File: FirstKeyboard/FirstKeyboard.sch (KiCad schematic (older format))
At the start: 24 parts, among them J1 USB_B_Mini, SW1 MXSwitch, SW2 MXSwitch, SW3 MXSwitch, SW4 MXSwitch, U1 ATmega32U4-AU, Y1 16MHz

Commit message: Last update of the day
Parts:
- C1, C2, C3, C4, C5, C6, C7, C8: footprint (none) -> Capacitor_SMD:C_0805_2012Metric_Pad1.15x1.40mm_HandSolder
- D1, D2, D3, D4: footprint (none) -> Diode_SMD:D_SOD-123
- J1: footprint (none) -> acheron_Connectors:USB_MiniB_XM7D-0512
- R1, R2, R3, R4: footprint (none) -> Resistor_SMD:R_1206_3216Metric_Pad1.42x1.75mm_HandSolder
- SW1, SW2, SW3, SW4: footprint (none) -> acheron_MX:MX100
- SWP1: footprint (none) -> acheron_Hardware:smdPushBtn
- Y1: footprint (none) -> Crystal:Crystal_SMD_5032-2Pin_5.0x3.2mm_HandSoldering
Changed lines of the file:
@@
 F 0 "SW1" H 7000 3000 50  0000 L CNN
 F 1 "MXSwitch" H 6950 2925 39  0000 L CNN
-F 2 "" H 7075 2925 50  0001 C CNN
+F 2 "acheron_MX:MX100" H 7075 2925 50  0001 C CNN
 F 3 "" H 7075 2925 50  0001 C CNN
 	1    7075 2925
@@
 F 0 "D1" V 7029 2543 50  0000 L CNN
 F 1 "D_Small" V 7120 2543 50  0000 L CNN
-F 2 "" V 7075 2475 50  0001 C CNN
+F 2 "Diode_SMD:D_SOD-123" V 7075 2475 50  0001 C CNN
 F 3 "~" V 7075 2475 50  0001 C CNN
 	1    7075 2475
@@
 F 0 "SW3" H 7925 3000 50  0000 L CNN
 F 1 "MXSwitch" H 7875 2925 39  0000 L CNN
-F 2 "" H 8000 2925 50  0001 C CNN
+F 2 "acheron_MX:MX100" H 8000 2925 50  0001 C CNN
 F 3 "" H 8000 2925 50  0001 C CNN
 	1    8000 2925
@@
 F 0 "D3" V 7954 2543 50  0000 L CNN
 F 1 "D_Small" V 8045 2543 50  0000 L CNN
-F 2 "" V 8000 2475 50  0001 C CNN
+F 2 "Diode_SMD:D_SOD-123" V 8000 2475 50  0001 C CNN
 F 3 "~" V 8000 2475 50  0001 C CNN
 	1    8000 2475
@@
 F 0 "SW4" H 7925 4275 50  0000 L CNN
 F 1 "MXSwitch" H 7875 4200 39  0000 L CNN
-F 2 "" H 8000 4200 50  0001 C CNN
+F 2 "acheron_MX:MX100" H 8000 4200 50  0001 C CNN
 F 3 "" H 8000 4200 50  0001 C CNN
 	1    8000 4200
@@
 F 0 "D4" V 7954 3818 50  0000 L CNN
 F 1 "D_Small" V 8045 3818 50  0000 L CNN
-F 2 "" V 8000 3750 50  0001 C CNN
+F 2 "Diode_SMD:D_SOD-123" V 8000 3750 50  0001 C CNN
 F 3 "~" V 8000 3750 50  0001 C CNN
 	1    8000 3750
@@
 F 0 "SW2" H 7000 4275 50  0000 L CNN
 F 1 "MXSwitch" H 6950 4200 39  0000 L CNN
-F 2 "" H 7075 4200 50  0001 C CNN
+F 2 "acheron_MX:MX100" H 7075 4200 50  0001 C CNN
 F 3 "" H 7075 4200 50  0001 C CNN
 	1    7075 4200
@@
 F 0 "D2" V 7029 3818 50  0000 L CNN
 F 1 "D_Small" V 7120 3818 50  0000 L CNN
-F 2 "" V 7075 3750 50  0001 C CNN
+F 2 "Diode_SMD:D_SOD-123" V 7075 3750 50  0001 C CNN
 F 3 "~" V 7075 3750 50  0001 C CNN
 	1    7075 3750
@@
 F 0 "R3" V 2604 5000 50  0000 C CNN
 F 1 "22R" V 2695 5000 50  0000 C CNN
-F 2 "" H 2800 5000 50  0001 C CNN
+F 2 "Resistor_SMD:R_1206_3216Metric_Pad1.42x1.75mm_HandSolder" H 2800 5000 50  0001 C CNN
 F 3 "~" H 2800 5000 50  0001 C CNN
 	1    2800 5000
@@
 F 0 "R2" V 2604 4900 50  0000 C CNN
 F 1 "22R" V 2695 4900 50  0000 C CNN
-F 2 "" H 2800 4900 50  0001 C CNN
+F 2 "Resistor_SMD:R_1206_3216Metric_Pad1.42x1.75mm_HandSolder" H 2800 4900 50  0001 C CNN
 F 3 "~" H 2800 4900 50  0001 C CNN
 	1    2800 4900
@@
 F 0 "J1" H 2150 5375 50  0000 C CNN
 F 1 "USB_B_Mini" H 2150 5275 50  0000 C CNN
-F 2 "" H 2300 4850 50  0001 C CNN
+F 2 "acheron_Connectors:USB_MiniB_XM7D-0512" H 2300 4850 50  0001 C CNN
 F 3 "~" H 2300 4850 50  0001 C CNN
 	1    2150 4900
@@
 F 0 "C5" V 3825 2575 50  0000 C CNN
 F 1 "10uF" V 3725 2575 50  0000 C CNN
-F 2 "" H 3625 2575 50  0001 C CNN
+F 2 "Capacitor_SMD:C_0805_2012Metric_Pad1.15x1.40mm_HandSolder" H 3625 2575 50  0001 C CNN
 F 3 "~" H 3625 2575 50  0001 C CNN
 	1    3625 2575
@@
 F 0 "C6" V 4125 2575 50  0000 C CNN
 F 1 "1uF" V 4025 2575 50  0000 C CNN
-F 2 "" H 3925 2575 50  0001 C CNN
+F 2 "Capacitor_SMD:C_0805_2012Metric_Pad1.15x1.40mm_HandSolder" H 3925 2575 50  0001 C CNN
 F 3 "~" H 3925 2575 50  0001 C CNN
 	1    3925 2575
@@
 F 0 "C7" V 4425 2575 50  0000 C CNN
 F 1 "100n" V 4325 2575 50  0000 C CNN
-F 2 "" H 4225 2575 50  0001 C CNN
+F 2 "Capacitor_SMD:C_0805_2012Metric_Pad1.15x1.40mm_HandSolder" H 4225 2575 50  0001 C CNN
 F 3 "~" H 4225 2575 50  0001 C CNN
 	1    4225 2575
@@
 F 0 "C8" V 4725 2575 50  0000 C CNN
 F 1 "100n" V 4625 2575 50  0000 C CNN
-F 2 "" H 4525 2575 50  0001 C CNN
+F 2 "Capacitor_SMD:C_0805_2012Metric_Pad1.15x1.40mm_HandSolder" H 4525 2575 50  0001 C CNN
 F 3 "~" H 4525 2575 50  0001 C CNN
 	1    4525 2575
@@
 F 0 "R1" H 2716 2854 50  0000 R CNN
 F 1 "10k" H 2716 2945 50  0000 R CNN
-F 2 "" H 2775 2900 50  0001 C CNN
+F 2 "Resistor_SMD:R_1206_3216Metric_Pad1.42x1.75mm_HandSolder" H 2775 2900 50  0001 C CNN
 F 3 "~" H 2775 2900 50  0001 C CNN
 	1    2775 2900
@@
 F 0 "SWP1" H 2700 3550 50  0000 R CNN
 F 1 "SW_Push" H 2725 3450 50  0000 R CNN
-F 2 "" H 2575 3400 50  0001 C CNN
+F 2 "acheron_Hardware:smdPushBtn" H 2575 3400 50  0001 C CNN
 F 3 "~" H 2575 3400 50  0001 C CNN
 	1    2575 3200
@@
 F 0 "C1" H 3025 3100 50  0000 R CNN
 F 1 "100n" H 3075 3300 50  0000 R CNN
-F 2 "" H 3075 3200 50  0001 C CNN
+F 2 "Capacitor_SMD:C_0805_2012Metric_Pad1.15x1.40mm_HandSolder" H 3075 3200 50  0001 C CNN
 F 3 "~" H 3075 3200 50  0001 C CNN
 	1    3075 3200
@@
 F 0 "R4" V 4729 6000 50  0000 C CNN
 F 1 "10k" V 4820 6000 50  0000 C CNN
-F 2 "" H 4925 6000 50  0001 C CNN
+F 2 "Resistor_SMD:R_1206_3216Metric_Pad1.42x1.75mm_HandSolder" H 4925 6000 50  0001 C CNN
 F 3 "~" H 4925 6000 50  0001 C CNN
 	1    4925 6000
@@
 F 0 "C3" V 2896 4300 50  0000 C CNN
 F 1 "22pF" V 2987 4300 50  0000 C CNN
-F 2 "" H 3125 4300 50  0001 C CNN
+F 2 "Capacitor_SMD:C_0805_2012Metric_Pad1.15x1.40mm_HandSolder" H 3125 4300 50  0001 C CNN
 F 3 "~" H 3125 4300 50  0001 C CNN
 	1    3125 4300
@@
 F 0 "C2" V 2975 4250 50  0000 C CNN
 F 1 "22pF" V 2987 4100 50  0000 C CNN
-F 2 "" H 3125 4100 50  0001 C CNN
+F 2 "Capacitor_SMD:C_0805_2012Metric_Pad1.15x1.40mm_HandSolder" H 3125 4100 50  0001 C CNN
 F 3 "~" H 3125 4100 50  0001 C CNN
 	1    3125 4100
@@
 F 0 "Y1" V 3225 4250 50  0000 R CNN
 F 1 "16MHz" V 3125 4300 50  0000 R CNN
-F 2 "" H 3375 4200 50  0001 C CNN
+F 2 "Crystal:Crystal_SMD_5032-2Pin_5.0x3.2mm_HandSoldering" H 3375 4200 50  0001 C CNN
 F 3 "~" H 3375 4200 50  0001 C CNN
 	1    3375 4200
@@
 F 0 "C4" V 3575 5200 50  0000 C CNN
 F 1 "1uF" V 3675 5200 50  0000 C CNN
-F 2 "" H 3425 5200 50  0001 C CNN
+F 2 "Capacitor_SMD:C_0805_2012Metric_Pad1.15x1.40mm_HandSolder" H 3425 5200 50  0001 C CNN
 F 3 "~" H 3425 5200 50  0001 C CNN
 	1    3425 5200

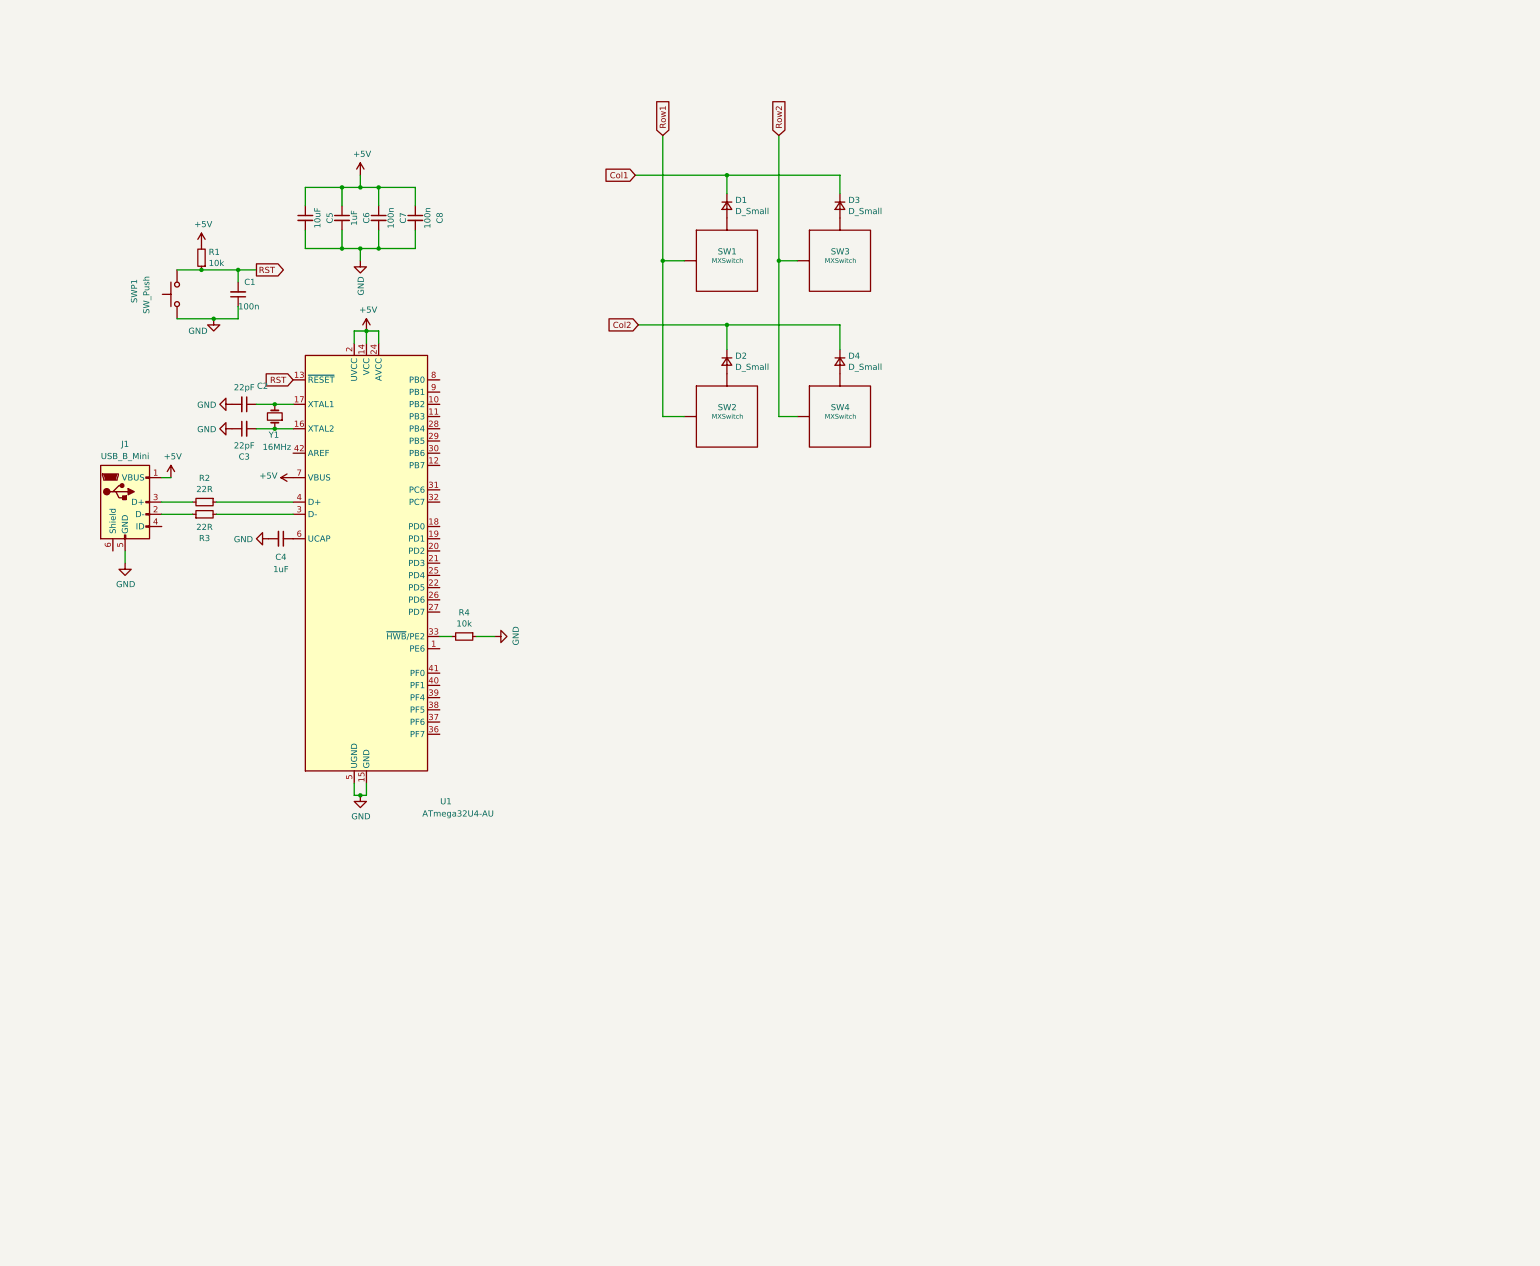
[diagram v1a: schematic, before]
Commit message: Dec10 Update, Starting full board
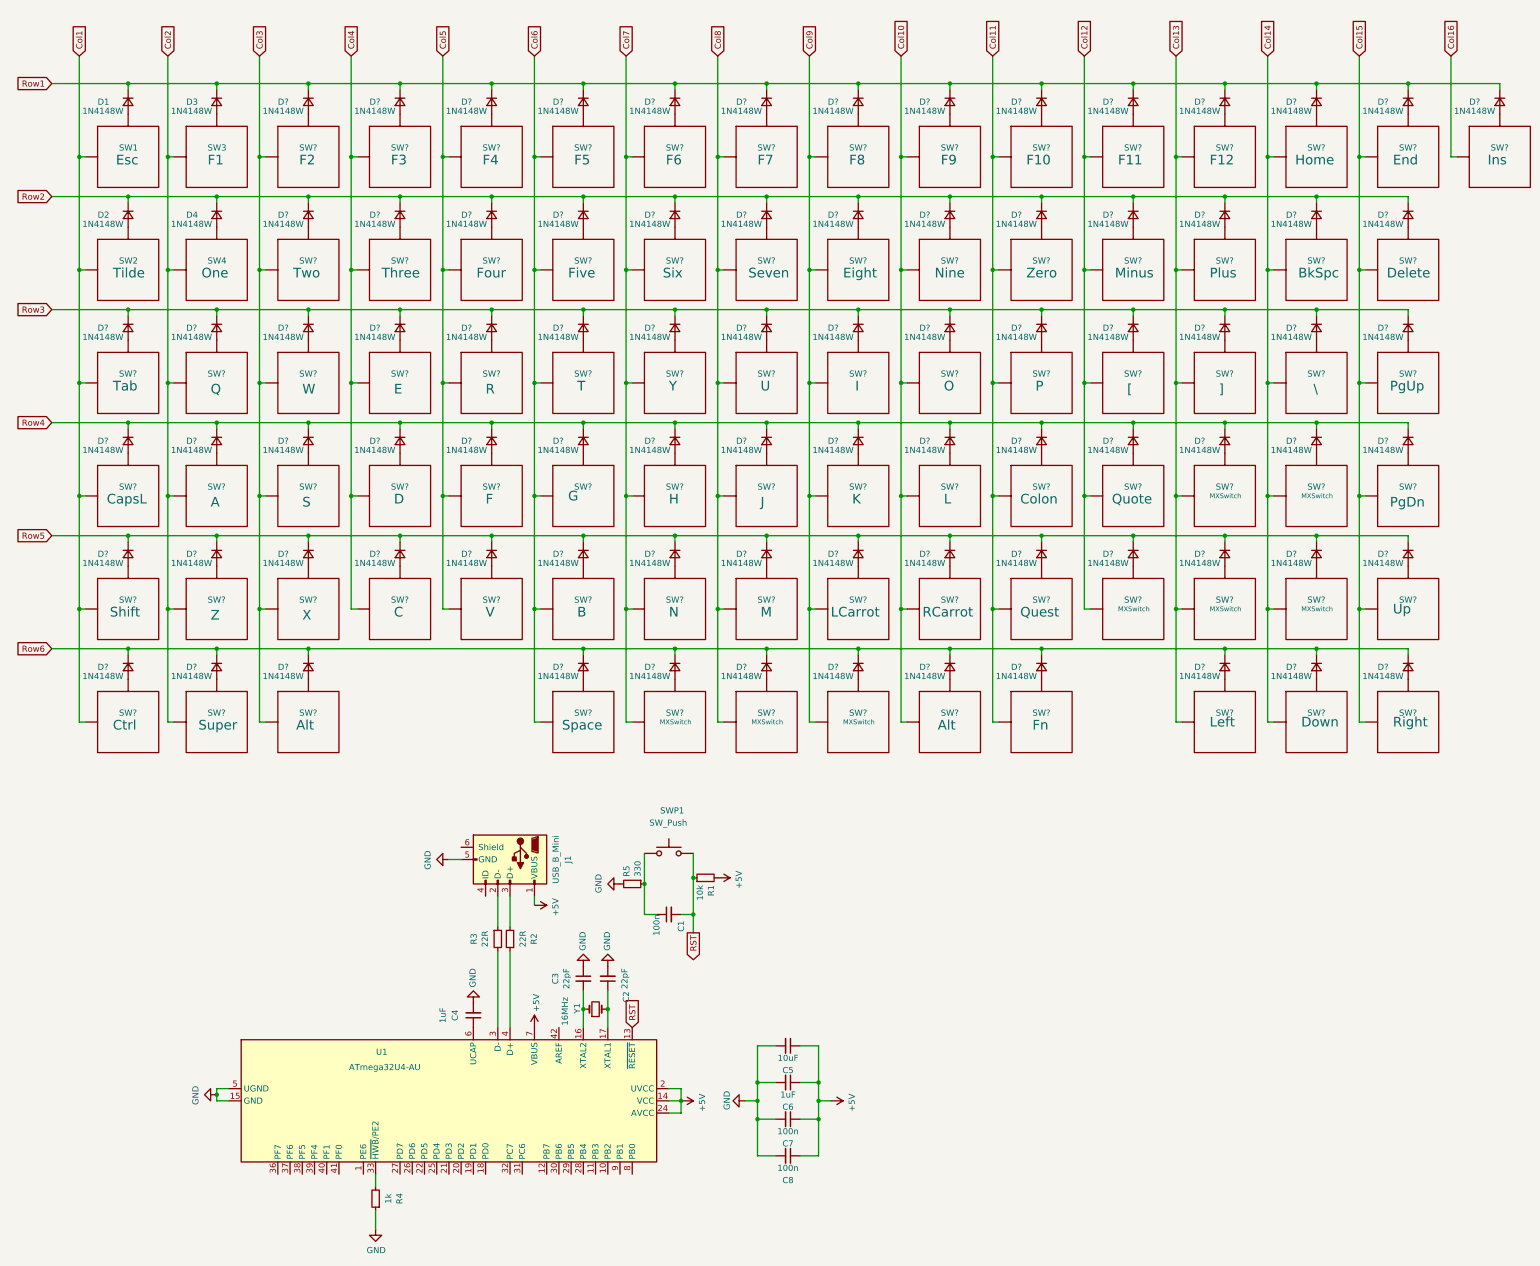
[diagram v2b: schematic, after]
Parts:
- added D? (x84): 1N4148W, Diode_SMD:D_SOD-123, symbol Device:D_Small
- added R5: 330, Resistor_SMD:R_1206_3216Metric_Pad1.42x1.75mm_HandSolder, symbol Device:R_Small
- added SW?: F2, acheron_MX:MX100, symbol acheronSymbols:MXSwitch
- added SW?: F3, acheron_MX:MX100, symbol acheronSymbols:MXSwitch
- added SW?: F4, acheron_MX:MX100, symbol acheronSymbols:MXSwitch
- added SW?: F5, acheron_MX:MX100, symbol acheronSymbols:MXSwitch
- added SW?: F6, acheron_MX:MX100, symbol acheronSymbols:MXSwitch
- added SW?: F7, acheron_MX:MX100, symbol acheronSymbols:MXSwitch
- added SW?: F8, acheron_MX:MX100, symbol acheronSymbols:MXSwitch
- added SW?: F9, acheron_MX:MX100, symbol acheronSymbols:MXSwitch
- added SW?: Ins, acheron_MX:MX100, symbol acheronSymbols:MXSwitch
- added SW?: End, acheron_MX:MX100, symbol acheronSymbols:MXSwitch
- added SW?: Home, acheron_MX:MX100, symbol acheronSymbols:MXSwitch
- added SW?: F12, acheron_MX:MX100, symbol acheronSymbols:MXSwitch
- added SW?: F11, acheron_MX:MX100, symbol acheronSymbols:MXSwitch
- added SW?: F10, acheron_MX:MX100, symbol acheronSymbols:MXSwitch
- added SW?: Two, acheron_MX:MX100, symbol acheronSymbols:MXSwitch
- added SW?: Nine, acheron_MX:MX100, symbol acheronSymbols:MXSwitch
- added SW?: Eight, acheron_MX:MX100, symbol acheronSymbols:MXSwitch
- added SW?: Seven, acheron_MX:MX100, symbol acheronSymbols:MXSwitch
- added SW?: Six, acheron_MX:MX100, symbol acheronSymbols:MXSwitch
- added SW?: Five, acheron_MX:MX100, symbol acheronSymbols:MXSwitch
- added SW?: Four, acheron_MX:MX100, symbol acheronSymbols:MXSwitch
- added SW?: Three, acheron_MX:MX100, symbol acheronSymbols:MXSwitch
- added SW?: Delete, acheron_MX:MX100, symbol acheronSymbols:MXSwitch
- added SW?: BkSpc, acheron_MX:MX100, symbol acheronSymbols:MXSwitch
- added SW?: Plus, acheron_MX:MX100, symbol acheronSymbols:MXSwitch
- added SW?: Minus, acheron_MX:MX100, symbol acheronSymbols:MXSwitch
- added SW?: Zero, acheron_MX:MX100, symbol acheronSymbols:MXSwitch
- added SW?: Tab, acheron_MX:MX100, symbol acheronSymbols:MXSwitch
- added SW?: Q, acheron_MX:MX100, symbol acheronSymbols:MXSwitch
- added SW?: CapsL, acheron_MX:MX100, symbol acheronSymbols:MXSwitch
- added SW?: A, acheron_MX:MX100, symbol acheronSymbols:MXSwitch
- added SW?: Shift, acheron_MX:MX100, symbol acheronSymbols:MXSwitch
- added SW?: Ctrl, acheron_MX:MX100, symbol acheronSymbols:MXSwitch
- added SW?: Super, acheron_MX:MX100, symbol acheronSymbols:MXSwitch
- added SW?: W, acheron_MX:MX100, symbol acheronSymbols:MXSwitch
- added SW?: O, acheron_MX:MX100, symbol acheronSymbols:MXSwitch
- added SW?: I, acheron_MX:MX100, symbol acheronSymbols:MXSwitch
- added SW?: U, acheron_MX:MX100, symbol acheronSymbols:MXSwitch
- added SW?: Y, acheron_MX:MX100, symbol acheronSymbols:MXSwitch
- added SW?: T, acheron_MX:MX100, symbol acheronSymbols:MXSwitch
- added SW?: R, acheron_MX:MX100, symbol acheronSymbols:MXSwitch
- added SW?: E, acheron_MX:MX100, symbol acheronSymbols:MXSwitch
- added SW?: PgUp, acheron_MX:MX100, symbol acheronSymbols:MXSwitch
- added SW?: \\, acheron_MX:MX100, symbol acheronSymbols:MXSwitch
- added SW?: ], acheron_MX:MX100, symbol acheronSymbols:MXSwitch
- added SW?: [, acheron_MX:MX100, symbol acheronSymbols:MXSwitch
- added SW?: P, acheron_MX:MX100, symbol acheronSymbols:MXSwitch
- added SW?: S, acheron_MX:MX100, symbol acheronSymbols:MXSwitch
- added SW?: L, acheron_MX:MX100, symbol acheronSymbols:MXSwitch
- added SW?: K, acheron_MX:MX100, symbol acheronSymbols:MXSwitch
- added SW?: J, acheron_MX:MX100, symbol acheronSymbols:MXSwitch
- added SW?: H, acheron_MX:MX100, symbol acheronSymbols:MXSwitch
- added SW?: G, acheron_MX:MX100, symbol acheronSymbols:MXSwitch
- added SW?: F, acheron_MX:MX100, symbol acheronSymbols:MXSwitch
- added SW?: D, acheron_MX:MX100, symbol acheronSymbols:MXSwitch
- added SW?: PgDn, acheron_MX:MX100, symbol acheronSymbols:MXSwitch
- added SW? (x8): MXSwitch, acheron_MX:MX100, symbol acheronSymbols:MXSwitch
- added SW?: Quote, acheron_MX:MX100, symbol acheronSymbols:MXSwitch
- added SW?: Colon, acheron_MX:MX100, symbol acheronSymbols:MXSwitch
- added SW?: X, acheron_MX:MX100, symbol acheronSymbols:MXSwitch
- added SW?: RCarrot, acheron_MX:MX100, symbol acheronSymbols:MXSwitch
- added SW?: LCarrot, acheron_MX:MX100, symbol acheronSymbols:MXSwitch
- added SW?: M, acheron_MX:MX100, symbol acheronSymbols:MXSwitch
- added SW?: N, acheron_MX:MX100, symbol acheronSymbols:MXSwitch
- added SW?: B, acheron_MX:MX100, symbol acheronSymbols:MXSwitch
- added SW?: V, acheron_MX:MX100, symbol acheronSymbols:MXSwitch
- added SW?: C, acheron_MX:MX100, symbol acheronSymbols:MXSwitch
- added SW?: Up, acheron_MX:MX100, symbol acheronSymbols:MXSwitch
- added SW?: Quest, acheron_MX:MX100, symbol acheronSymbols:MXSwitch
- added SW? (x2): Alt, acheron_MX:MX100, symbol acheronSymbols:MXSwitch
- added SW?: Space, acheron_MX:MX100, symbol acheronSymbols:MXSwitch
- added SW?: Right, acheron_MX:MX100, symbol acheronSymbols:MXSwitch
- added SW?: Down, acheron_MX:MX100, symbol acheronSymbols:MXSwitch
- added SW?: Left, acheron_MX:MX100, symbol acheronSymbols:MXSwitch
- added SW?: Fn, acheron_MX:MX100, symbol acheronSymbols:MXSwitch
- added SW?: Z, acheron_MX:MX100, symbol acheronSymbols:MXSwitch
- D1, D2, D3, D4: value D_Small -> 1N4148W
- R4: value 10k -> 1k
- SW1: value MXSwitch -> Esc
- SW2: value MXSwitch -> Tilde
- SW3: value MXSwitch -> F1
- SW4: value MXSwitch -> One
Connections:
- net Col1: now also SW1.1 (Col), SW2.1 (Col), SW?.1 (Col), SW?.1 (Col), SW?.1 (Col), SW?.1 (Col); no longer D1.1 (K), D3.1 (K)
- net Col2: now also SW3.1 (Col), SW4.1 (Col), SW?.1 (Col), SW?.1 (Col), SW?.1 (Col), SW?.1 (Col); no longer D2.1 (K), D4.1 (K)
- net GND: now also R5.2; no longer C1.1, SWP1.1
- net Row1: now also D1.1 (K), D3.1 (K), D?.1 (K), D?.1 (K), D?.1 (K), D?.1 (K), D?.1 (K), D?.1 (K), D?.1 (K), D?.1 (K), D?.1 (K), D?.1 (K), D?.1 (K), D?.1 (K), D?.1 (K), D?.1 (K); no longer SW1.1 (Col), SW2.1 (Col)
- net Row2: now also D2.1 (K), D4.1 (K), D?.1 (K), D?.1 (K), D?.1 (K), D?.1 (K), D?.1 (K), D?.1 (K), D?.1 (K), D?.1 (K), D?.1 (K), D?.1 (K), D?.1 (K), D?.1 (K), D?.1 (K); no longer SW3.1 (Col), SW4.1 (Col)
- new net: C1.1, R5.1, SWP1.1
- new net: D?.2 (A), SW?.2 (Row) (x84)
- new net Col10: SW?.1 (Col), SW?.1 (Col), SW?.1 (Col), SW?.1 (Col), SW?.1 (Col), SW?.1 (Col)
- new net Col11: SW?.1 (Col), SW?.1 (Col), SW?.1 (Col), SW?.1 (Col), SW?.1 (Col), SW?.1 (Col)
- new net Col12: SW?.1 (Col), SW?.1 (Col), SW?.1 (Col), SW?.1 (Col), SW?.1 (Col)
- new net Col13: SW?.1 (Col), SW?.1 (Col), SW?.1 (Col), SW?.1 (Col), SW?.1 (Col), SW?.1 (Col)
- new net Col14: SW?.1 (Col), SW?.1 (Col), SW?.1 (Col), SW?.1 (Col), SW?.1 (Col), SW?.1 (Col)
- new net Col15: SW?.1 (Col), SW?.1 (Col), SW?.1 (Col), SW?.1 (Col), SW?.1 (Col), SW?.1 (Col)
- new net Col16: SW?.1 (Col)
- new net Col3: SW?.1 (Col), SW?.1 (Col), SW?.1 (Col), SW?.1 (Col), SW?.1 (Col), SW?.1 (Col)
- new net Col4: SW?.1 (Col), SW?.1 (Col), SW?.1 (Col), SW?.1 (Col), SW?.1 (Col)
- new net Col5: SW?.1 (Col), SW?.1 (Col), SW?.1 (Col), SW?.1 (Col), SW?.1 (Col)
- new net Col6: SW?.1 (Col), SW?.1 (Col), SW?.1 (Col), SW?.1 (Col), SW?.1 (Col), SW?.1 (Col)
- new net Col7: SW?.1 (Col), SW?.1 (Col), SW?.1 (Col), SW?.1 (Col), SW?.1 (Col), SW?.1 (Col)
- new net Col8: SW?.1 (Col), SW?.1 (Col), SW?.1 (Col), SW?.1 (Col), SW?.1 (Col), SW?.1 (Col)
- new net Col9: SW?.1 (Col), SW?.1 (Col), SW?.1 (Col), SW?.1 (Col), SW?.1 (Col), SW?.1 (Col)
- new net Row3: D?.1 (K), D?.1 (K), D?.1 (K), D?.1 (K), D?.1 (K), D?.1 (K), D?.1 (K), D?.1 (K), D?.1 (K), D?.1 (K), D?.1 (K), D?.1 (K), D?.1 (K), D?.1 (K), D?.1 (K)
- new net Row4: D?.1 (K), D?.1 (K), D?.1 (K), D?.1 (K), D?.1 (K), D?.1 (K), D?.1 (K), D?.1 (K), D?.1 (K), D?.1 (K), D?.1 (K), D?.1 (K), D?.1 (K), D?.1 (K), D?.1 (K)
- new net Row5: D?.1 (K), D?.1 (K), D?.1 (K), D?.1 (K), D?.1 (K), D?.1 (K), D?.1 (K), D?.1 (K), D?.1 (K), D?.1 (K), D?.1 (K), D?.1 (K), D?.1 (K), D?.1 (K), D?.1 (K)
- new net Row6: D?.1 (K), D?.1 (K), D?.1 (K), D?.1 (K), D?.1 (K), D?.1 (K), D?.1 (K), D?.1 (K), D?.1 (K), D?.1 (K), D?.1 (K), D?.1 (K)
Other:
- moved on the sheet: C1, C2, C3, C4, C5, C6, C7, C8, D1, D2, D3, D4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
